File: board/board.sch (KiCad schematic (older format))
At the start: 13 parts, among them J1 ESP-01, J2 Conn_01x05, J3 Conn_01x02, J4 Conn_02x02_Counter_Clockwise, J5 Conn_01x03

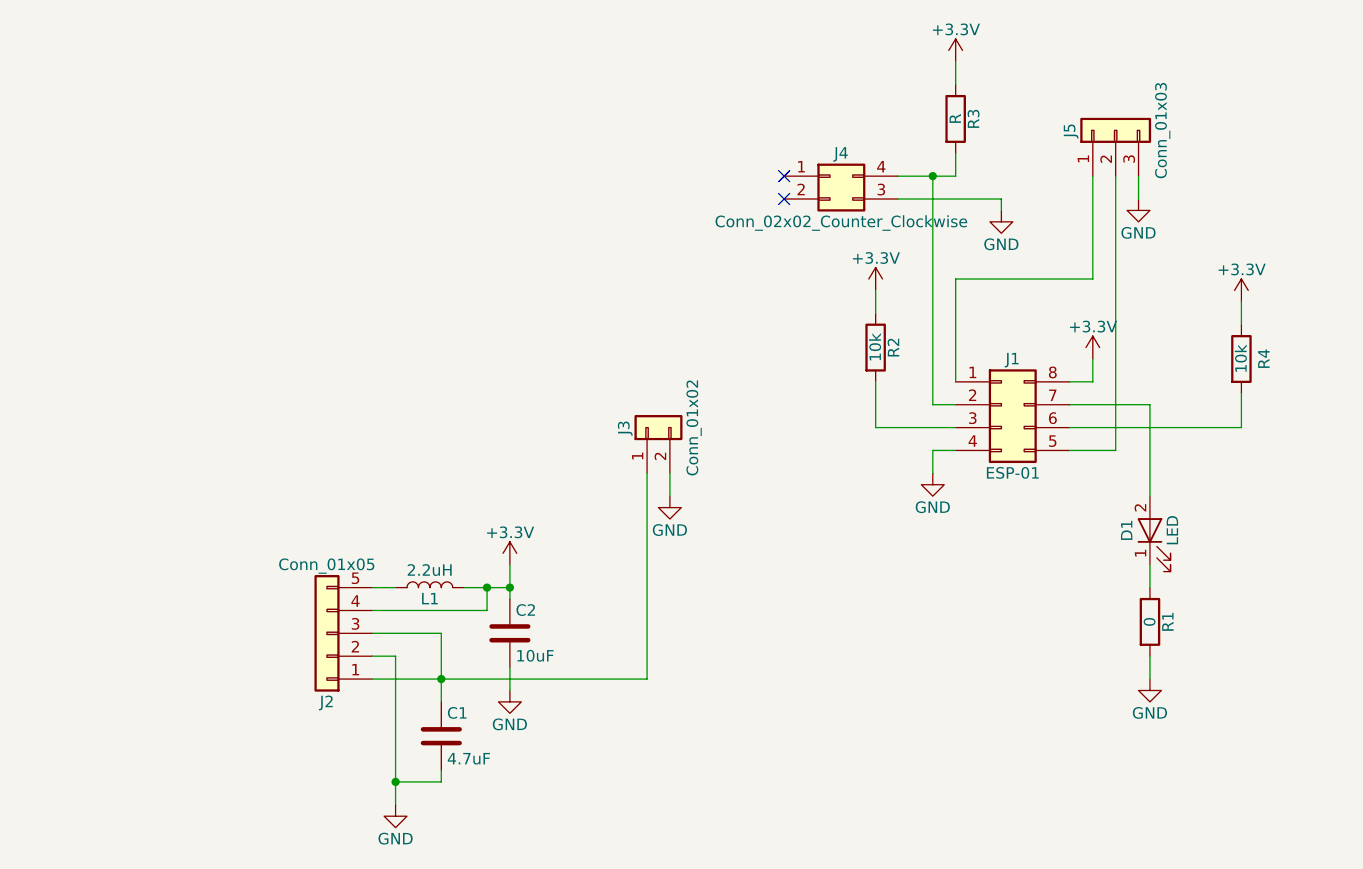
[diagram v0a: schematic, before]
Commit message: Updated schematic
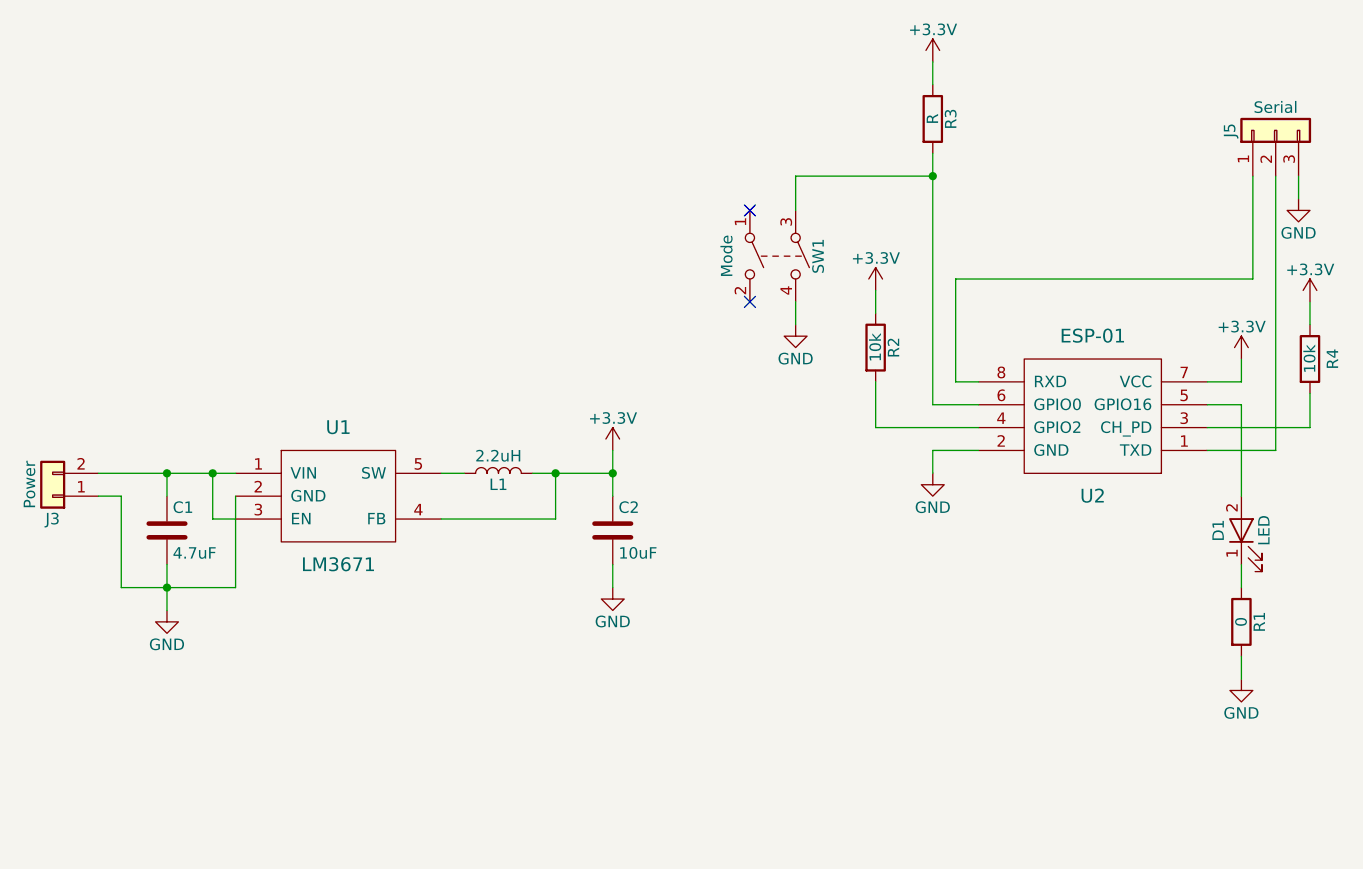
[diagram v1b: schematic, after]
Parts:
- removed J1: ESP-01, symbol Conn_02x04_Counter_Clockwise
- removed J2: Conn_01x05, TO_SOT_Packages_SMD:SOT-23-5, symbol Conn_01x05
- removed J4: Conn_02x02_Counter_Clockwise, symbol Conn_02x02_Counter_Clockwise
- added SW1: Mode, nebrius-switch:KMR641NG, symbol SW_DPST
- added U1: LM3671, TO_SOT_Packages_SMD:SOT-23-5_HandSoldering, symbol LM3671
- added U2: ESP-01, Pin_Headers:Pin_Header_Straight_2x04_Pitch2.54mm, symbol ESP-01
- D1: footprint (none) -> Resistors_SMD:R_0805_HandSoldering
- J3: value Conn_01x02 -> Power
- J5: value Conn_01x03 -> Serial
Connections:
- net +3V3: now also U1.4 (FB), U2.7 (VCC)
- net GND: now also J3.1 (Pin_1), SW1.4, U1.2 (GND), U2.2 (GND); no longer J3.2 (Pin_2)
- net at J5.1 (Pin_1): now also U2.8 (RXD)
- net at R3.2: now also SW1.3, U2.6 (GPIO0)
- net at R2.2: now also U2.4 (GPIO2)
- net at J5.2 (Pin_2): now also U2.1 (TXD)
- net at R4.2: now also U2.3 (CH_PD)
- net at D1.2 (A): now also U2.5 (GPIO16)
- net at C1.1: now also J3.2 (Pin_2), U1.1 (VIN), U1.3 (EN); no longer J3.1 (Pin_1)
- net at L1.1: now also U1.5 (SW)
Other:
- moved on the sheet: C1, D1, J3, J5, L1, R1, R3, R4
